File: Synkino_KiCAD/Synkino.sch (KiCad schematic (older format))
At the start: 60 parts

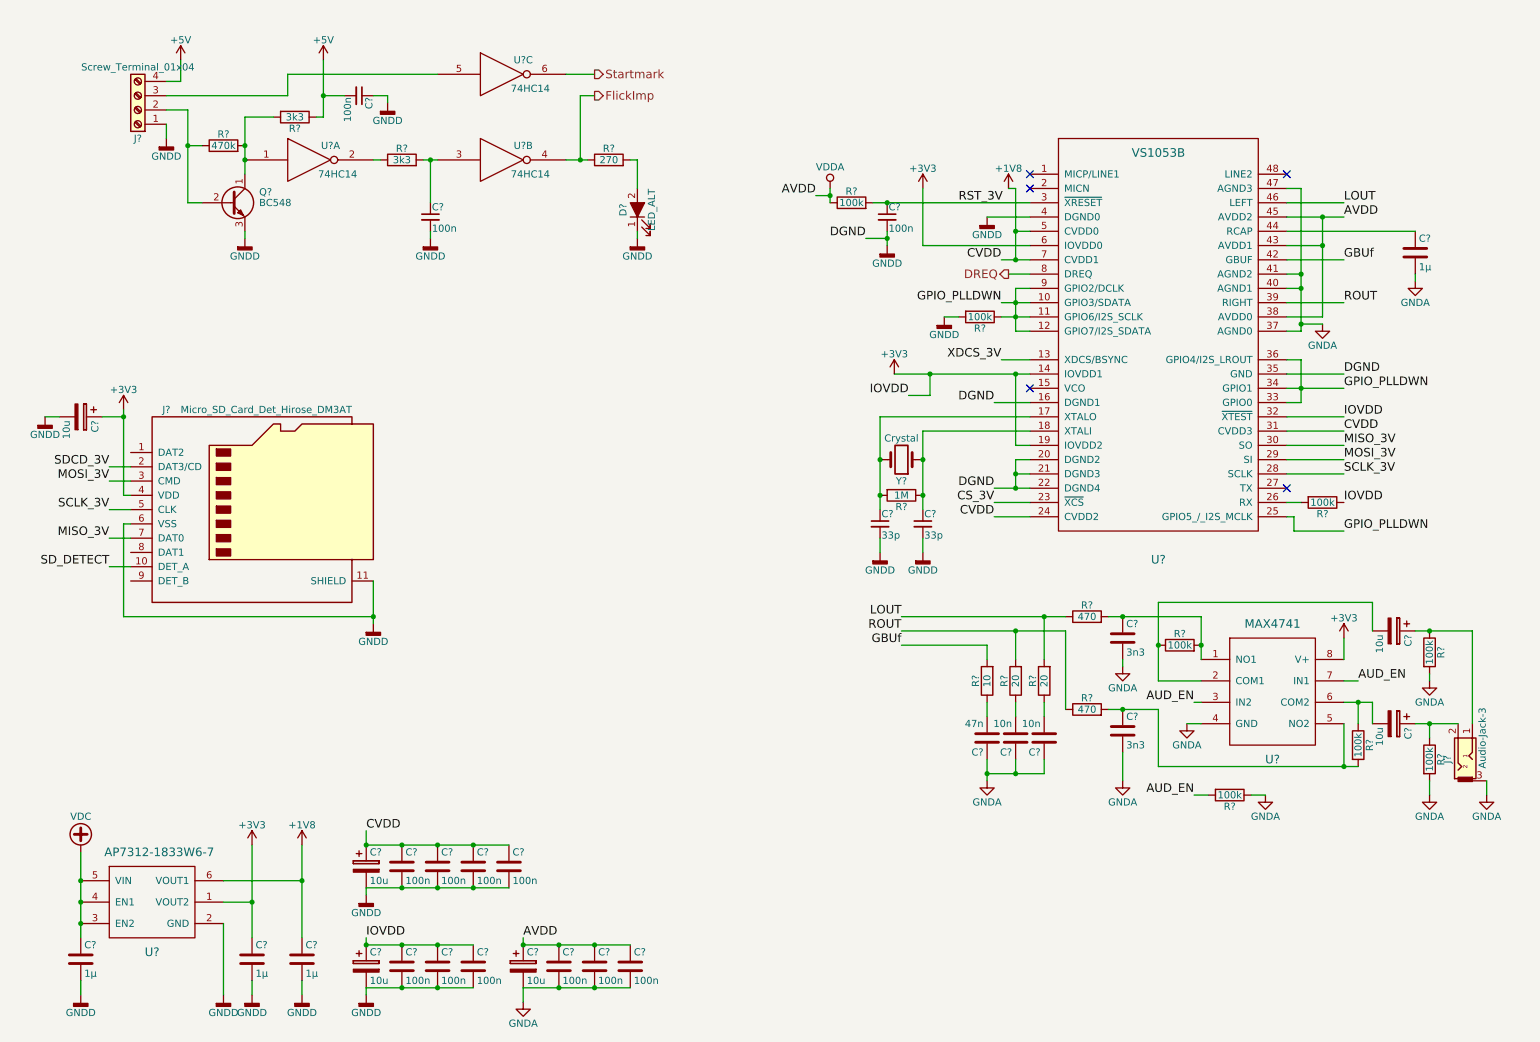
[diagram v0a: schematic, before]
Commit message: Schematics Progress
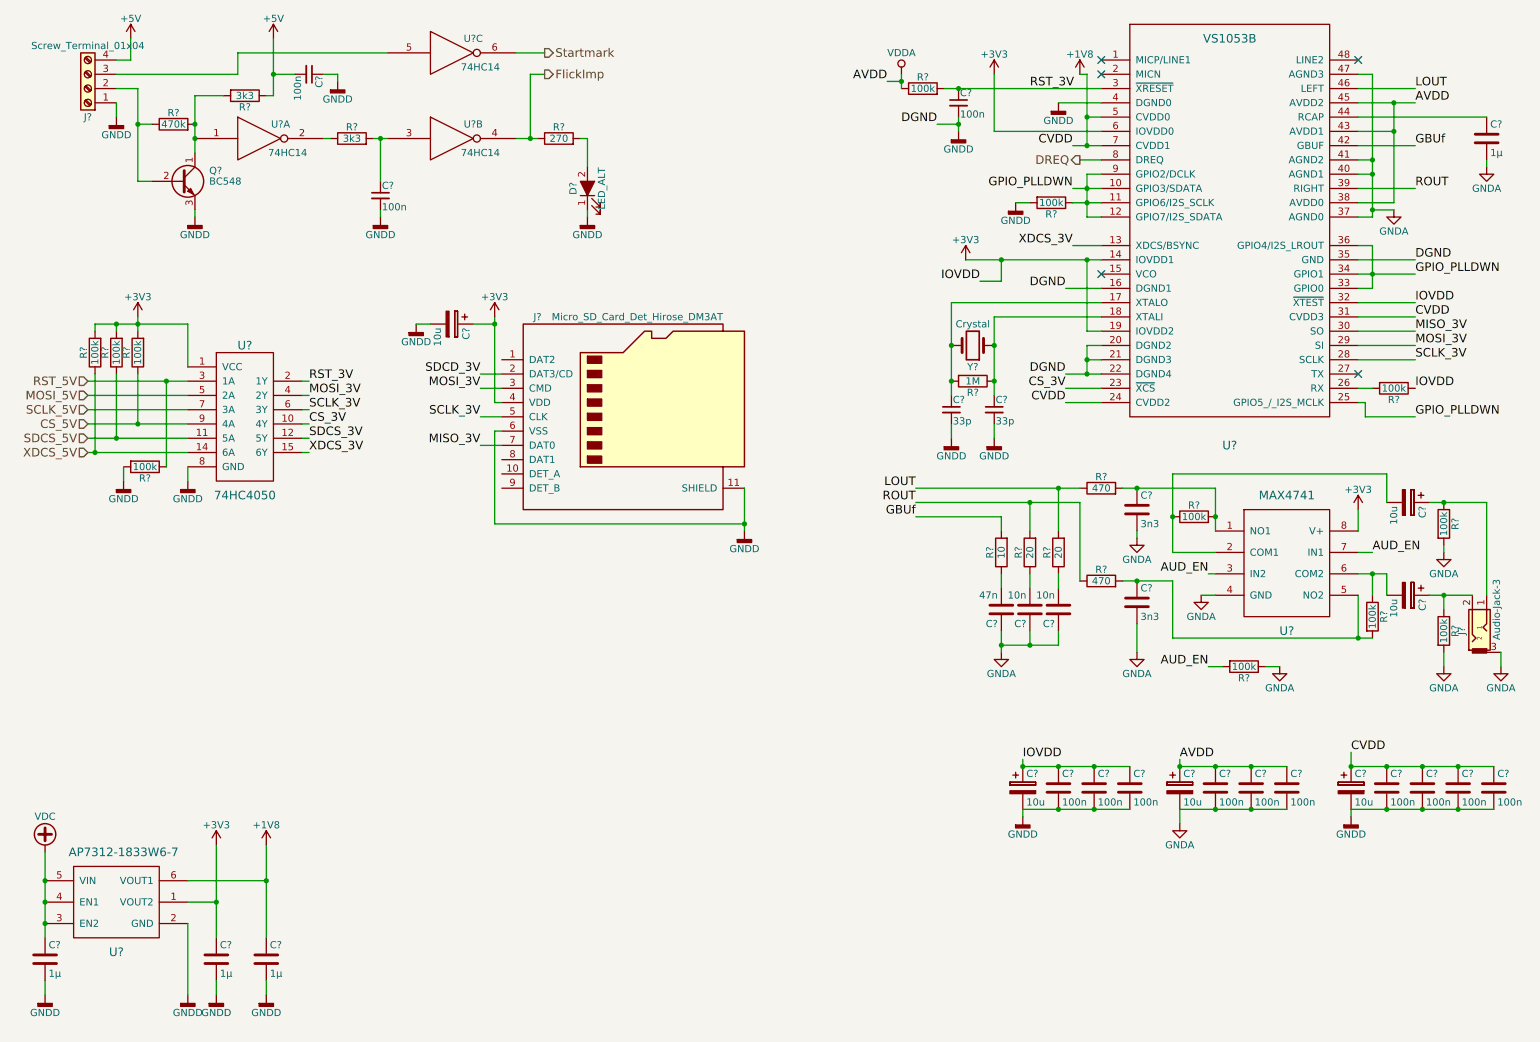
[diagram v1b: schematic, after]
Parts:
- added R? (x4): 100k, symbol R
- added U?: 74HC4050, symbol 74HC4050
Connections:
- net +3V3: now also R?.2, R?.2, R?.2, U?.1 (VCC)
- net CS_3V: now also U?.10 (4Y)
- net GNDD: now also R?.2, U?.8 (GND)
- net MOSI_3V: now also U?.4 (2Y)
- net RST_3V: now also U?.2 (1Y)
- net SCLK_3V: now also U?.6 (3Y)
- net XDCS_3V: now also U?.15 (6Y)
- net SD_DETECT: no longer names the net of J?.10 (DET_A)
- new net CS_5V: R?.1, U?.9 (4A)
- new net MOSI_5V: U?.5 (2A)
- new net RST_5V: R?.1, U?.3 (1A)
- new net SCLK_5V: U?.7 (3A)
- new net SDCS_3V: U?.12 (5Y)
- new net SDCS_5V: R?.1, U?.11 (5A)
- new net XDCS_5V: R?.1, U?.14 (6A)
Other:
- moved on the sheet: C?, D?, J?, Q?, R?, U?, U?A, U?B, U?C, Y?
